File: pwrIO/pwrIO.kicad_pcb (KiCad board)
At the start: 4 copper layers, 33.7 x 30.3 mm, 55 parts, among them IC3 TLV61225DC, J1 MOTOR1, J2 MOTOR2, J3 VCC_MOTOR, J4 MOTOR1, J5 MOTOR2, J6 MISC, J7 ENC1, J8 ENC2, U1 TB6612FNG, U2 TB6612FNG

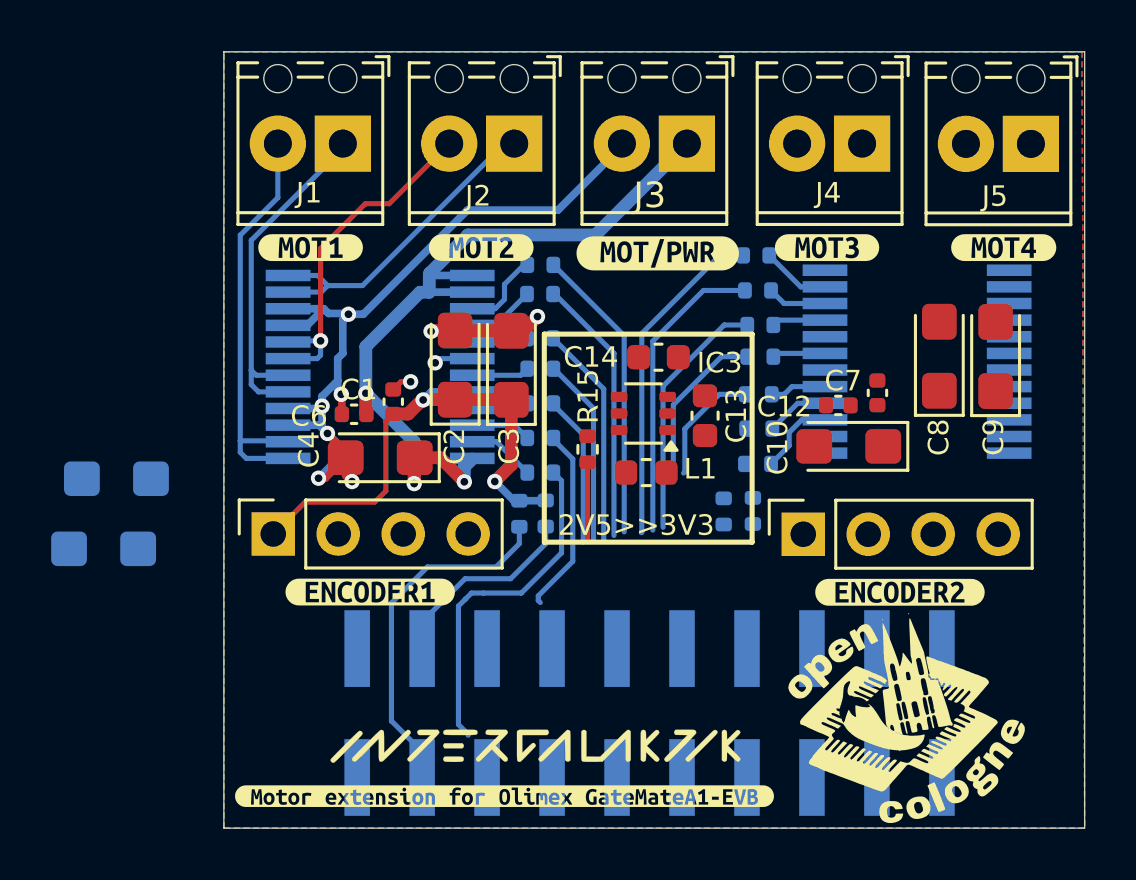
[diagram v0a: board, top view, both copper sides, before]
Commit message: sch pcb
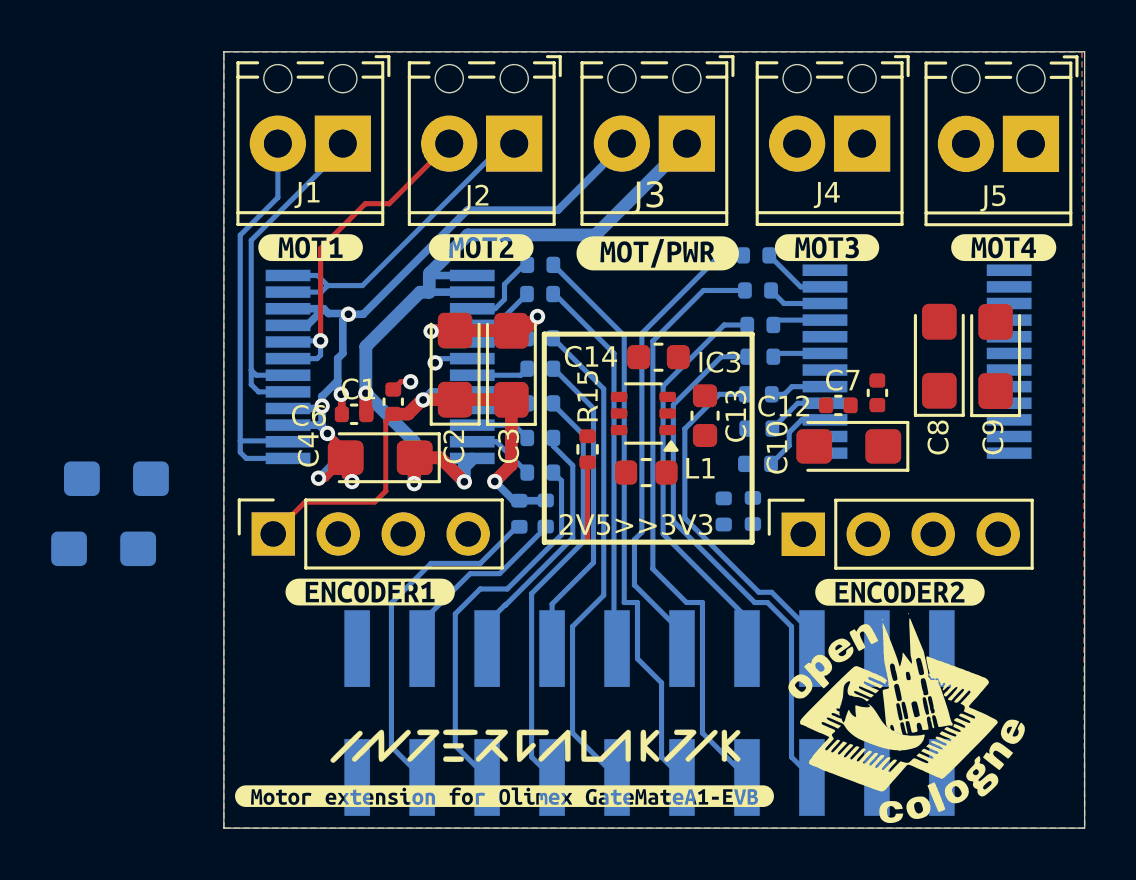
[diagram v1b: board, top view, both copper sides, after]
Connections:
- R1 pad 1: /MOTOR_1/STBY -> /NB_B2
- R10 pad 1: /NB_B2 -> /MOTOR_2/PWMB
- R11 pad 1: /NB_B3 -> /NB_B5
- R12 pad 1: /NB_B4 -> /NB_A5
- R13 pad 1: /NB_B5 -> /NB_B6
- R14 pad 1: /NB_B6 -> /MOTOR_2/BIN2
- R2 pad 1: /NB_A1 -> /MOTOR_1/PWMA
- R3 pad 1: /NB_A2 -> /NB_A4
- R4 pad 1: /NB_A3 -> /NB_A2
- R5 pad 1: /NB_A4 -> /NB_B1
- R6 pad 1: /NB_A5 -> /NB_A3
- R7 pad 1: /NB_A6 -> /NB_B3
- R8 pad 1: /MOTOR_2/STBY -> /NB_A6
- R9 pad 1: /NB_B1 -> /NB_B4
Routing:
- net /NB_A4: track 7.34 -> 22.4 mm
- net /NB_A5: track 8.73 -> 23.4 mm
- net /NB_B6: track 0.00 -> 13.9 mm
- net /NB_A3: track 5.92 -> 19.2 mm
- net /NB_B2: track 0.00 -> 12.3 mm
- net /NB_B5: track 4.69 -> 15.9 mm
- net /NB_A6: track 10.5 -> 20.8 mm
- net /MOTOR_1/STBY: track 7.36 -> 0.00 mm
- net /NB_B4: track 11.8 -> 18.5 mm
- net /MOTOR_2/STBY: track 6.65 -> 0.00 mm
- net /NB_B3: track 9.80 -> 14.9 mm
- net /NB_A2: track 11.6 -> 16.3 mm
- net /NB_B1: track 13.0 -> 10.2 mm
- net /NB_A1: track 13.4 -> 14.9 mm
